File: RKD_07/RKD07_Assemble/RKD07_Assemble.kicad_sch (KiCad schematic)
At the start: 147 parts, among them J1 Conn_01x02_Socket, J2 Conn_01x24, J3 Conn_01x24, J4 Conn_01x24, SW1 SW_Push, SW10 SW_Push, SW11 SW_Push, SW12 SW_Push, SW13 SW_Push, SW14 SW_Push, SW15 SW_Push, SW16 SW_Push, SW17 SW_Push, SW18 SW_Push, SW19 SW_Push, SW2 SW_Push, SW20 SW_Push, SW21 SW_Push, SW22 SW_Push, SW23 SW_Push, SW24 SW_Push, SW25 SW_Push, SW26 SW_Push, SW27 SW_Push, SW28 SW_Push, SW29 SW_Push, SW3 SW_Push, SW30 RotaryEncoder_Switch, SW31 SW_Push, SW4 SW_Push, SW5 SW_Push, SW51 SW_Push, SW52 SW_Push, SW53 SW_Push, SW54 SW_Push, SW55 SW_Push, SW56 SW_Push, SW57 SW_Push, SW58 SW_Push, SW59 SW_Push, SW6 SW_Push, SW60 SW_Push, SW61 SW_Push, SW62 SW_Push, SW63 SW_Push, SW64 SW_Push, SW65 SW_Push, SW66 SW_Push, SW67 SW_Push, SW68 SW_Push, SW69 SW_Push, SW7 SW_Push, SW70 SW_Push, SW71 SW_Push, SW72 SW_Push, SW73 SW_Push, SW74 SW_Push, SW75 SW_Push, SW76 SW_Push, SW77 SW_Push, SW78 SW_Push, SW79 SW_Push, SW8 SW_Push, SW80 SW_Push, SW81 SW_Push, SW82 SW_Push, SW83 SW_Push, SW84 SW_Push, SW85 SW_Push, SW86 SW_Push, SW87 SW_Push, SW88 SW_Push, SW89 SW_Push, SW9 SW_Push, SW90 SW_Push, U1 Pico

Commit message: RKD07 一時保存
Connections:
- net GP18_R is gone; now on net SDA/SCK_R: J3.14 (Pin_14), J4.11 (Pin_11)
- net GP19_R is gone; now on net SCL/TX_R: J3.13 (Pin_13), J4.12 (Pin_12)
- net GND_L: now also U1.23 (GND)
- net SCL/TX_L: now also J2.12 (Pin_12), U1.25 (GPIO19); no longer J2.1 (Pin_1), U1.20 (GPIO15)
- net SCL/TX_R: no longer J3.24 (Pin_24), J4.1 (Pin_1)
- net SDA/SCK_L: now also J2.11 (Pin_11), U1.24 (GPIO18); no longer J2.2 (Pin_2), U1.19 (GPIO14)
- net SDA/SCK_R: no longer J3.23 (Pin_23), J4.2 (Pin_2)
- new net GP14_R: J3.23 (Pin_23), J4.2 (Pin_2)
- new net GP15_R: J3.24 (Pin_24), J4.1 (Pin_1)
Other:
- note added: "GND VCC 3V3 GP28 GP27 GP26 GP25 GP24 GP23 GP22 GP21 GP20 GP19 GP18 GP17 GP16 GP08 GP09 GP10 GP11 GP12 GP13 GP14 GP15"
- moved on the sheet: J2

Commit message: RD07配線
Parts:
- added J10, J9: Conn_01x04, Connector_PinSocket_2.54mm:PinSocket_1x04_P2.54mm_Horizontal, symbol Connector_Generic:Conn_01x04
- added J5, J6: Qwiic_RA, SparkFun-Connector:JST_SMD_1.0mm-4_Black, symbol SparkFun-Connector:Qwiic_Right_Angle
- added J7, J8: Conn_01x06, Connector_FFC-FPC:Hirose_FH12-6S-0.5SH_1x06-1MP_P0.50mm_Horizontal, symbol Connector_Generic:Conn_01x06
- added R1, R2: R, Resistor_THT:R_Axial_DIN0207_L6.3mm_D2.5mm_P10.16mm_Horizontal, symbol Device:R
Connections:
- net GP12_R is gone; now on net ROW1_R: J3.21 (Pin_21), J4.4 (Pin_4)
- net GP13_R is gone; now on net ROW2_R: J3.22 (Pin_22), J4.3 (Pin_3)
- net GP14_R is gone; now on net ROW3_R: J3.23 (Pin_23), J4.2 (Pin_2)
- net GP15_R is gone; now on net ROW4_R: J3.24 (Pin_24), J4.1 (Pin_1)
- net GP20_R is gone; now on net COL6_R: J3.12 (Pin_12), J4.13 (Pin_13)
- net GP21_R is gone; now on net COL7_R: J3.11 (Pin_11), J4.14 (Pin_14)
- net GP22_R is gone; now on net COL8_R: J3.10 (Pin_10), J4.15 (Pin_15)
- net GP23_R is gone; now on net COL9_R: J3.9 (Pin_9), J4.16 (Pin_16)
- net GP24_R is gone; now on net COL10_R: J3.8 (Pin_8), J4.17 (Pin_17)
- net GP25_R is gone; now on net COL11_R: J3.7 (Pin_7), J4.18 (Pin_18)
- net GP26_R is gone; now on net COL12_R: J3.6 (Pin_6), J4.19 (Pin_19)
- net GP27_R is gone; now on net COL13_R: J3.5 (Pin_5), J4.20 (Pin_20)
- net GP28_R is gone; now on net ROW0_R: J3.4 (Pin_4), J4.21 (Pin_21)
- net 3v3_L: now also J5.2 (Pin_2), J8.6 (Pin_6)
- net 3v3_R: now also J6.2 (Pin_2), J7.6 (Pin_6), J9.2 (Pin_2), J9.3 (Pin_3), R1.1, R2.1
- net COL0_L: now also J2.10 (Pin_10), U1.2 (GPIO1)
- net COL1_L: now also J2.9 (Pin_9), U1.4 (GPIO2)
- net COL2_L: now also J2.8 (Pin_8), U1.5 (GPIO3)
- net COL3_L: now also J2.7 (Pin_7), U1.6 (GPIO4)
- net COL4_L: now also J2.6 (Pin_6), U1.7 (GPIO5)
- net COL5_L: now also J2.5 (Pin_5), U1.9 (GPIO6)
- net GND_L: now also U1.28 (GND), J5.1 (Pin_1), J8.1 (Pin_1), J8.5 (Pin_5)
- net GND_R: now also J6.1 (Pin_1), J7.1 (Pin_1), J7.5 (Pin_5)
- net RE_A: now also U1.15 (GPIO11), J10.1 (Pin_1)
- net RE_B: now also U1.16 (GPIO12), J10.4 (Pin_4)
- net ROW0_L: now also J2.21 (Pin_21), U1.1 (GPIO0)
- net ROW1_L: now also J2.4 (Pin_4), U1.10 (GPIO7)
- net ROW2_L: now also J2.3 (Pin_3), U1.11 (GPIO8)
- net ROW3_L: now also J2.2 (Pin_2), U1.12 (GPIO9)
- net ROW4_L: now also J2.1 (Pin_1), U1.14 (GPIO10)
- net SCL/TX_L: now also J10.3 (Pin_3), J5.4 (Pin_4)
- net SCL/TX_R: now also J6.4 (Pin_4), J7.3 (Pin_3), J9.1 (Pin_1), R1.2
- net SDA/SCK_L: now also J10.2 (Pin_2), J5.3 (Pin_3)
- net SDA/SCK_R: now also J6.3 (Pin_3), J7.2 (Pin_2), J9.4 (Pin_4), R2.2
- net SCK_L: now reaches U1.19 (GPIO14)
- net SCK_L: now also J8.2 (Pin_2)
- net TX_L: now reaches U1.20 (GPIO15)
- net TX_L: now also J8.3 (Pin_3)
- net COL6_L: now reaches U1.21 (GPIO16)
- net COL6_L: now also J2.13 (Pin_13)
- net COL7_L: now reaches U1.22 (GPIO17)
- net COL7_L: now also J2.14 (Pin_14)
- net COL8_L: now reaches U1.26 (GPIO20)
- net COL8_L: now also J2.15 (Pin_15)
- net COL9_L: now reaches U1.27 (GPIO21)
- net COL9_L: now also J2.16 (Pin_16)
- net COL10_L: now reaches U1.29 (GPIO22)
- net COL10_L: now also J2.17 (Pin_17)
- net COL11_L: now reaches U1.31 (GPIO26_ADC0)
- net COL11_L: now also J2.18 (Pin_18)
- net COL12_L: now reaches U1.32 (GPIO27_ADC1)
- net COL12_L: now also J2.19 (Pin_19)
- net COL13_L: now reaches U1.34 (GPIO28_ADC2)
- net COL13_L: now also J2.20 (Pin_20)
- net GP08_R renamed COL2_R
- net GP09_R renamed COL3_R
- net GP10_R renamed COL4_R
- net GP11_R renamed COL5_R
- net GP16_R renamed COL1_R
- net GP17_R renamed COL0_R
- no-connect marks 8 -> 15
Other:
- note added: "CS"
- note added: "MOTION"
- note added: "Resist for i2c"

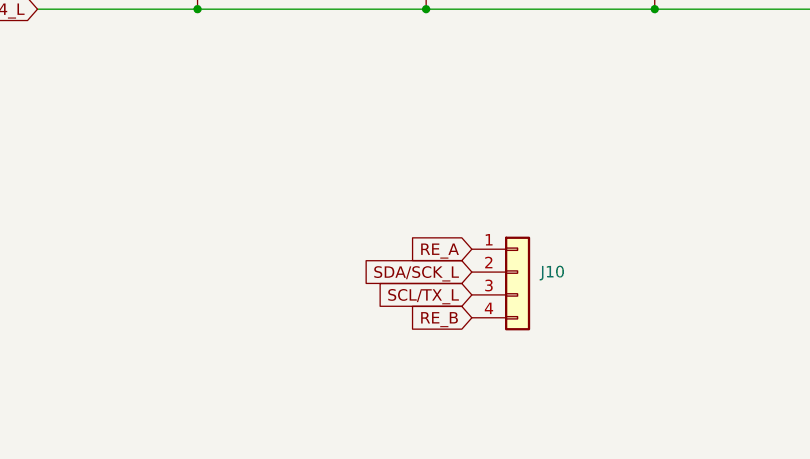
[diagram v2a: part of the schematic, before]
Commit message: 07 Modify
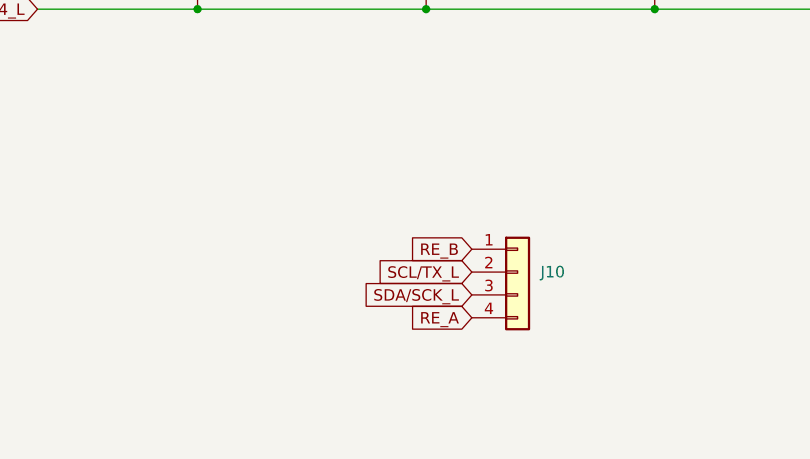
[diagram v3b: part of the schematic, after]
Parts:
- J10: footprint Connector_PinSocket_2.54mm:PinSocket_1x04_P2.54mm_Horizontal -> Connector_PinHeader_2.54mm:PinHeader_1x04_P2.54mm_Horizontal
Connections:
- net RE_A: now also J10.4 (Pin_4); no longer J10.1 (Pin_1)
- net RE_B: now also J10.1 (Pin_1); no longer J10.4 (Pin_4)
- net SCL/TX_L: now also J10.2 (Pin_2); no longer J10.3 (Pin_3)
- net SDA/SCK_L: now also J10.3 (Pin_3); no longer J10.2 (Pin_2)
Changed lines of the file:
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@@
 		)
 	)
-	(global_label "COL7_L"
+	(global_label "SCL{slash}TX_L"
 		(shape input)
-		(at 90.17 100.33 0)
+		(at 88.9 386.08 180)
 		(fields_autoplaced yes)
 		(effects
@@
 				(size 1.27 1.27)
 			)
-			(justify left)
+			(justify right)
 		)
 		(property "Intersheetrefs" "${INTERSHEET_REFS}"
-			(at 99.989 100.33 0)
+			(at 76.9039 386.08 0)
 			(effects
 				(font
 					(size 1.27 1.27)
 				)
-				(justify left)
+				(justify right)
 				(hide yes)
 			)
 		)
 	)
-	(global_label "SDA{slash}SCK_L"
+	(global_label "COL7_L"
 		(shape input)
-		(at 88.9 386.08 180)
+		(at 90.17 100.33 0)
 		(fields_autoplaced yes)
 		(effects
@@
 				(size 1.27 1.27)
 			)
-			(justify right)
+			(justify left)
 		)
 		(property "Intersheetrefs" "${INTERSHEET_REFS}"
-			(at 75.271 386.08 0)
+			(at 99.989 100.33 0)
 			(effects
 				(font
 					(size 1.27 1.27)
 				)
-				(justify right)
+				(justify left)
 				(hide yes)
 			)
@@
 		)
 	)
-	(global_label "RE_B"
-		(shape input)
-		(at 88.9 391.16 180)
-		(fields_autoplaced yes)
-		(effects
-			(font
-				(size 1.27 1.27)
-			)
-			(justify right)
-		)
-		(property "Intersheetrefs" "${INTERSHEET_REFS}"
-			(at 81.2582 391.16 0)
-			(effects
-				(font
-					(size 1.27 1.27)
-				)
-				(justify right)
-				(hide yes)
-			)
-		)
-	)
 	(global_label "COL9_R"
 		(shape input)
@@
 		)
 	)
+	(global_label "SDA{slash}SCK_L"
+		(shape input)
+		(at 88.9 388.62 180)
+		(fields_autoplaced yes)
+		(effects
+			(font
+				(size 1.27 1.27)
+			)
+			(justify right)
+		)
+		(property "Intersheetrefs" "${INTERSHEET_REFS}"
+			(at 75.271 388.62 0)
+			(effects
+				(font
+					(size 1.27 1.27)
+				)
+				(justify right)
+				(hide yes)
+			)
+		)
+	)
 	(global_label "ROW4_L"
 		(shape input)
@@
 		)
 	)
-	(global_label "RE_A"
-		(shape input)
-		(at 88.9 383.54 180)
-		(fields_autoplaced yes)
-		(effects
-			(font
-				(size 1.27 1.27)
-			)
-			(justify right)
-		)
-		(property "Intersheetrefs" "${INTERSHEET_REFS}"
-			(at 81.4396 383.54 0)
-			(effects
-				(font
-					(size 1.27 1.27)
-				)
-				(justify right)
-				(hide yes)
-			)
-		)
-	)
 	(global_label "SCL{slash}TX_L"
 		(shape input)
@@
 		)
 	)
-	(global_label "SCL{slash}TX_L"
+	(global_label "RE_A"
 		(shape input)
-		(at 259.08 157.48 0)
+		(at 88.9 391.16 180)
 		(fields_autoplaced yes)
 		(effects
@@
 				(size 1.27 1.27)
 			)
-			(justify left)
+			(justify right)
 		)
 		(property "Intersheetrefs" "${INTERSHEET_REFS}"
-			(at 271.0761 157.48 0)
+			(at 81.4396 391.16 0)
 			(effects
 				(font
 					(size 1.27 1.27)
 				)
-				(justify left)
+				(justify right)
 				(hide yes)
 			)
 		)
 	)
-	(global_label "COL0_L"
+	(global_label "SCL{slash}TX_L"
 		(shape input)
-		(at 259.08 162.56 0)
+		(at 259.08 157.48 0)
 		(fields_autoplaced yes)
 		(effects
@@
 		)
 		(property "Intersheetrefs" "${INTERSHEET_REFS}"
-			(at 268.899 162.56 0)
+			(at 271.0761 157.48 0)
 			(effects
 				(font
@@
 		)
 	)
-	(global_label "COL12_R"
+	(global_label "COL0_L"
 		(shape input)
-		(at 292.1 139.7 180)
+		(at 259.08 162.56 0)
 		(fields_autoplaced yes)
 		(effects
@@
 				(size 1.27 1.27)
 			)
-			(justify right)
+			(justify left)
 		)
 		(property "Intersheetrefs" "${INTERSHEET_REFS}"
-			(at 280.8296 139.7 0)
+			(at 268.899 162.56 0)
 			(effects
 				(font
 					(size 1.27 1.27)
 				)
-				(justify right)
+				(justify left)
 				(hide yes)
 			)
 		)
 	)
-	(global_label "RE_B"
+	(global_label "COL12_R"
 		(shape input)
-		(at 134.62 381 180)
+		(at 292.1 139.7 180)
 		(fields_autoplaced yes)
 		(effects
@@
 		)
 		(property "Intersheetrefs" "${INTERSHEET_REFS}"
-			(at 126.9782 381 0)
+			(at 280.8296 139.7 0)
 			(effects
 				(font
@@
 		)
 	)
-	(global_label "SCL{slash}TX_L"
+	(global_label "RE_B"
 		(shape input)
-		(at 88.9 388.62 180)
+		(at 134.62 381 180)
 		(fields_autoplaced yes)
 		(effects
@@
 		)
 		(property "Intersheetrefs" "${INTERSHEET_REFS}"
-			(at 76.9039 388.62 0)
+			(at 126.9782 381 0)
 			(effects
 				(font
@@
 		)
 	)
+	(global_label "RE_B"
+		(shape input)
+		(at 88.9 383.54 180)
+		(fields_autoplaced yes)
+		(effects
+			(font
+				(size 1.27 1.27)
+			)
+			(justify right)
+		)
+		(property "Intersheetrefs" "${INTERSHEET_REFS}"
+			(at 81.2582 383.54 0)
+			(effects
+				(font
+					(size 1.27 1.27)
+				)
+				(justify right)
+				(hide yes)
+			)
+		)
+	)
 	(global_label "COL9_L"
 		(shape input)
@@
 			)
 		)
-		(property "Footprint" "Connector_PinSocket_2.54mm:PinSocket_1x04_P2.54mm_Horizontal"
+		(property "Footprint" "Connector_PinHeader_2.54mm:PinHeader_1x04_P2.54mm_Horizontal"
 			(at 93.98 386.08 0)
 			(effects
